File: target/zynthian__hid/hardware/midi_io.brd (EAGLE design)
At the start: 70 x 25 mm, 5 parts, among them IC1 74AC00N, IC2 74AC00N

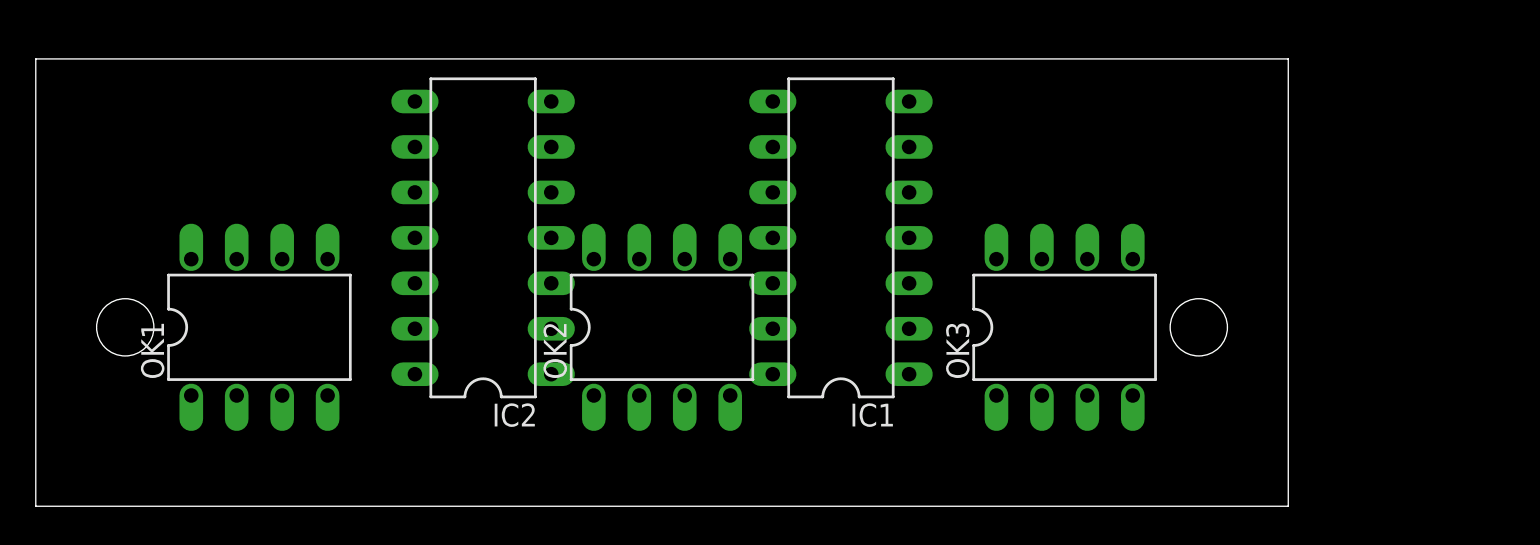
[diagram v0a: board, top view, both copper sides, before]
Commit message: zynthian__hid: updated hardware
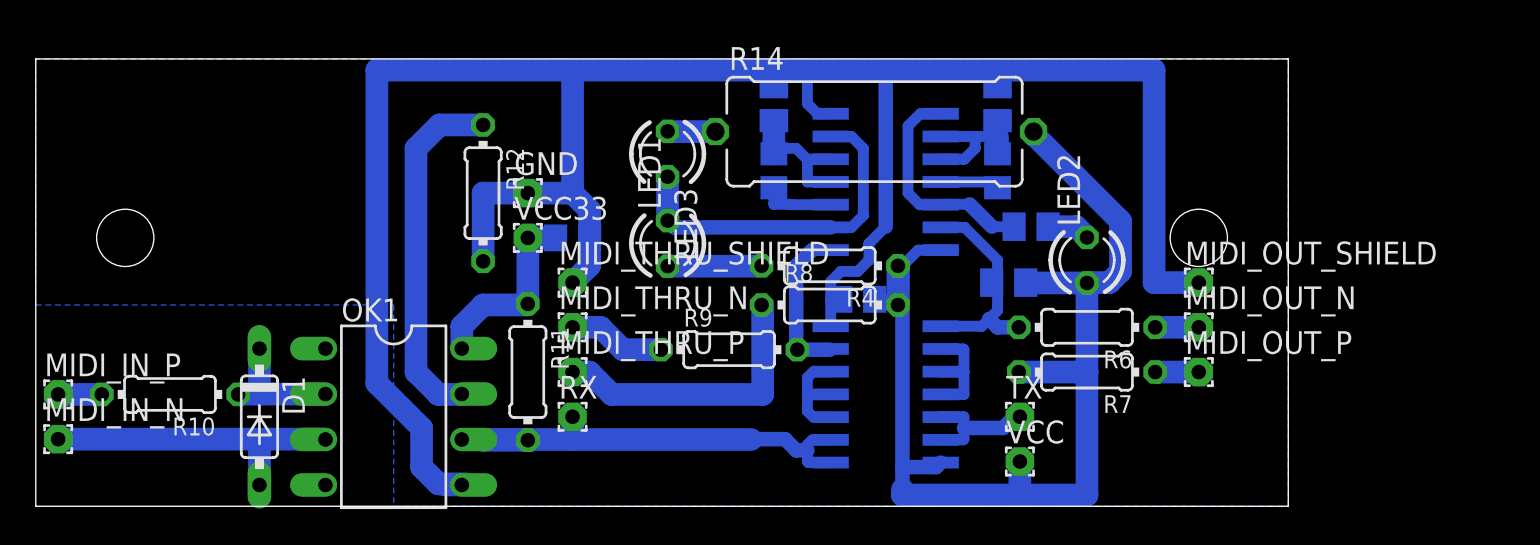
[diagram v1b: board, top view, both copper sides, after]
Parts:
- removed OK2, OK3: 6N137, optocoupler:DIL08
- added C1, C2: 1uF, rcl:C0805
- added C3, C4: 0.1, rcl:C0805
- added D1: 1N4148DO35-7, diode:DO35-7
- added GND, MIDI_IN_N, MIDI_IN_P, MIDI_OUT_N, MIDI_OUT_P, MIDI_OUT_SHIELD, MIDI_THRU_N, MIDI_THRU_P, MIDI_THRU_SHIELD, RX, TX, VCC, VCC33: (no value), wirepad:1,6/0,8
- added LED1, LED2, LED3: (no value), led:LED3MM
- added R1, R2: 1M, rcl:M0805
- added R10, R4, R6, R7, R8, R9: 220, rcl:0204/7
- added R11: 1K, rcl:0204/7
- added R12: 4K7, rcl:0204/7
- added R14: 220, rcl:0617/17
- added R3: 100k, rcl:M0805
- added R5: 220, rcl:M0805
- IC1, IC2: value 74AC00N -> 74AC00D; device 74xx-eu:DIL14 -> 74xx-eu:SO14
- moved IC2 24.1 mm to (47.5, 6.25), flipped to the bottom
- moved OK1 9.01 mm to (20.0, 5.00), turned to 270 degrees
- moved IC1 4.00 mm to (47.5, 18.1), flipped to the bottom
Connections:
- new net INV1: IC2.3, IC2.4, IC2.5
- new net INV2: IC2.10, IC2.11, IC2.9
- new net L2: LED2.K, R5.1
- new net LED_MIDI_IN_THRU: IC1.2, IC1.6, LED1.K, LED3.K
- new net LED_MIDI_OUT: IC1.12, IC1.8, R5.2
- new net MIDI_THRU_N: MIDI_THRU_N.1, R9.1
- new net MIDI_THRU_P: MIDI_THRU_P.1, R8.1
- new net MIDI_TX_N: MIDI_OUT_N.1, R6.1
- new net MIDI_TX_P: MIDI_OUT_P.1, R7.1
- new net MO: IC1.13, IC2.8, R3.1, R6.2
- new net N$1: OK1.7, R12.1
- new net N$2: LED1.A, R4.2
- new net N$4: LED3.A, R14.1
- new net N$5: D1.C, OK1.2, R10.1
- new net N$6: D1.A, MIDI_IN_N.1, OK1.3
- new net N$7: MIDI_IN_P.1, R10.2
- new net RC1: C1.2, IC1.4, IC1.5, R1.2
- new net RC2: C2.2, IC1.10, IC1.9, R2.2
- new net RX: IC2.1, IC2.2, OK1.6, R11.2, RX.1
- new net THRU: IC1.1, IC2.6, R9.2
- new net TO_C1: C1.1, IC1.3
- new net TO_C2: C2.1, IC1.11
- new net TX: IC2.12, IC2.13, TX.1
- new net VCC33: C4.2, OK1.8, R11.1, VCC33.1
- net GND: now also C3.1, C4.1, GND.1, MIDI_OUT_SHIELD.1, MIDI_THRU_SHIELD.1, OK1.5, R1.1, R12.2, R2.1
- net VCC: now also C3.2, LED2.A, R14.2, R3.2, R4.1, R7.2, R8.2, VCC.1
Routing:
- net GND: track 0.00 -> 128.7 mm
- net VCC: track 0.00 -> 65.4 mm
- net RX: track 0.00 -> 27.0 mm
- net N$1: track 0.00 -> 19.9 mm
- net LED_MIDI_IN_THRU: track 0.00 -> 19.7 mm
- net N$6: track 0.00 -> 17.5 mm
- net MIDI_THRU_P: track 0.00 -> 16.2 mm
- net LED_MIDI_OUT: track 0.00 -> 12.6 mm
- net MO: track 0.00 -> 12.4 mm
- net VCC33: track 0.00 -> 10.7 mm
- net RC2: track 0.00 -> 9.14 mm
- net THRU: track 0.00 -> 8.92 mm
- net RC1: track 0.00 -> 8.43 mm
- net N$5: track 0.00 -> 7.43 mm
- net TX: track 0.00 -> 7.26 mm
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- added copper zone on layer 16, net GND
